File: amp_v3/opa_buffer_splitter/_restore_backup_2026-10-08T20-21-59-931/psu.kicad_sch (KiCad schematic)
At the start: 20 parts, among them J1 UHP_PWR, J2 PWR_OUT_VA, J3 PWR_OUT_VA, J4 PWR_OUT_VA, J5 PWR_OUT_VA, U1 DPB09B-12

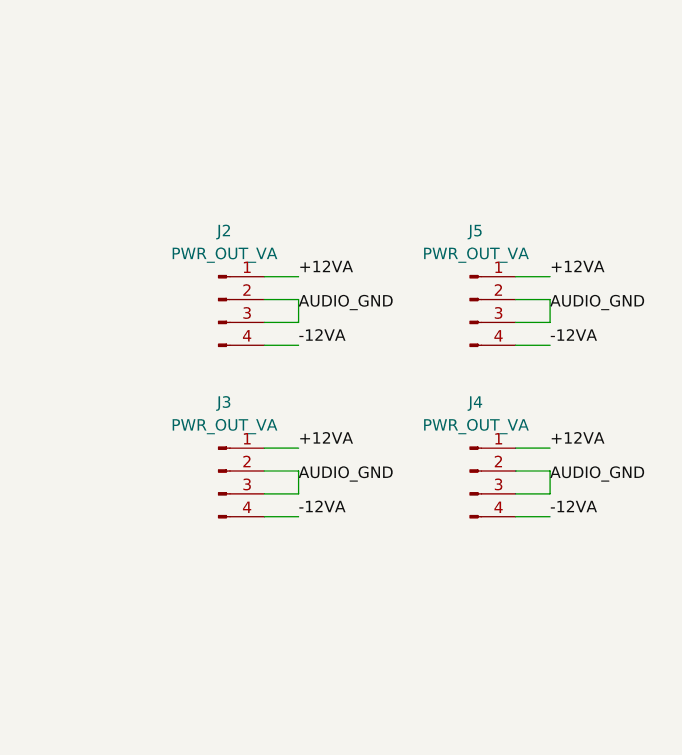
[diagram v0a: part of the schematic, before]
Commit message: updates
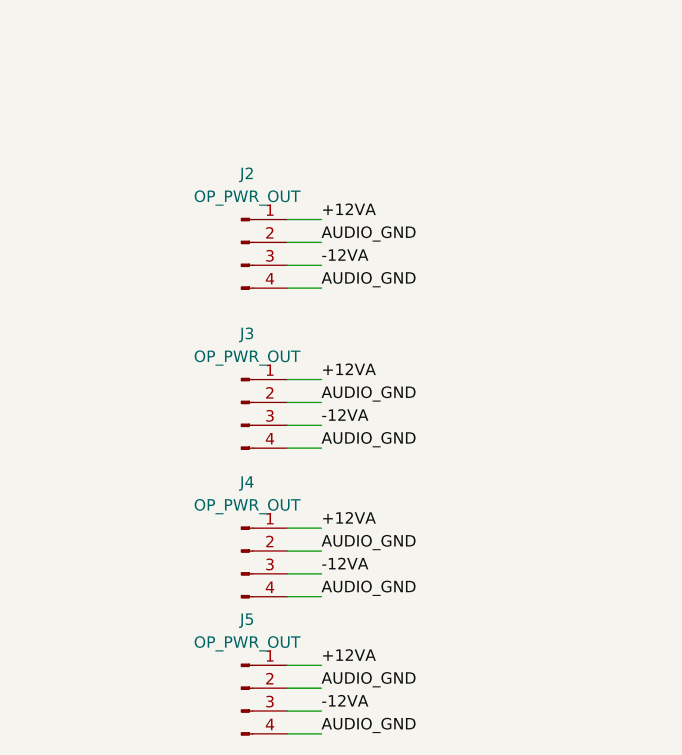
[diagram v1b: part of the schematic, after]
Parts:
- J2, J3, J4, J5: value PWR_OUT_VA -> OP_PWR_OUT
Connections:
- net -12VA: now also J2.3 (Pin_3), J3.3 (Pin_3), J4.3 (Pin_3), J5.3 (Pin_3); no longer J2.4 (Pin_4), J3.4 (Pin_4), J4.4 (Pin_4), J5.4 (Pin_4)
- net AUDIO_GND: now also J2.4 (Pin_4), J3.4 (Pin_4), J4.4 (Pin_4), J5.4 (Pin_4); no longer J2.3 (Pin_3), J3.3 (Pin_3), J4.3 (Pin_3), J5.3 (Pin_3)
